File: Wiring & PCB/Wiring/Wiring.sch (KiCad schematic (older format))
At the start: 24 parts, among them M0 Motor_DC, M1 Motor_DC, M2 Stepper_Motor_unipolar_6pin, SW0 Ascention Limit 1, SW1 Ascention Limit 2, SW2 Declination Limit 1, U0 Arduino-mega, U1 Ardunio_Micro, U3 ULN2004A, U4 pchero_dualH

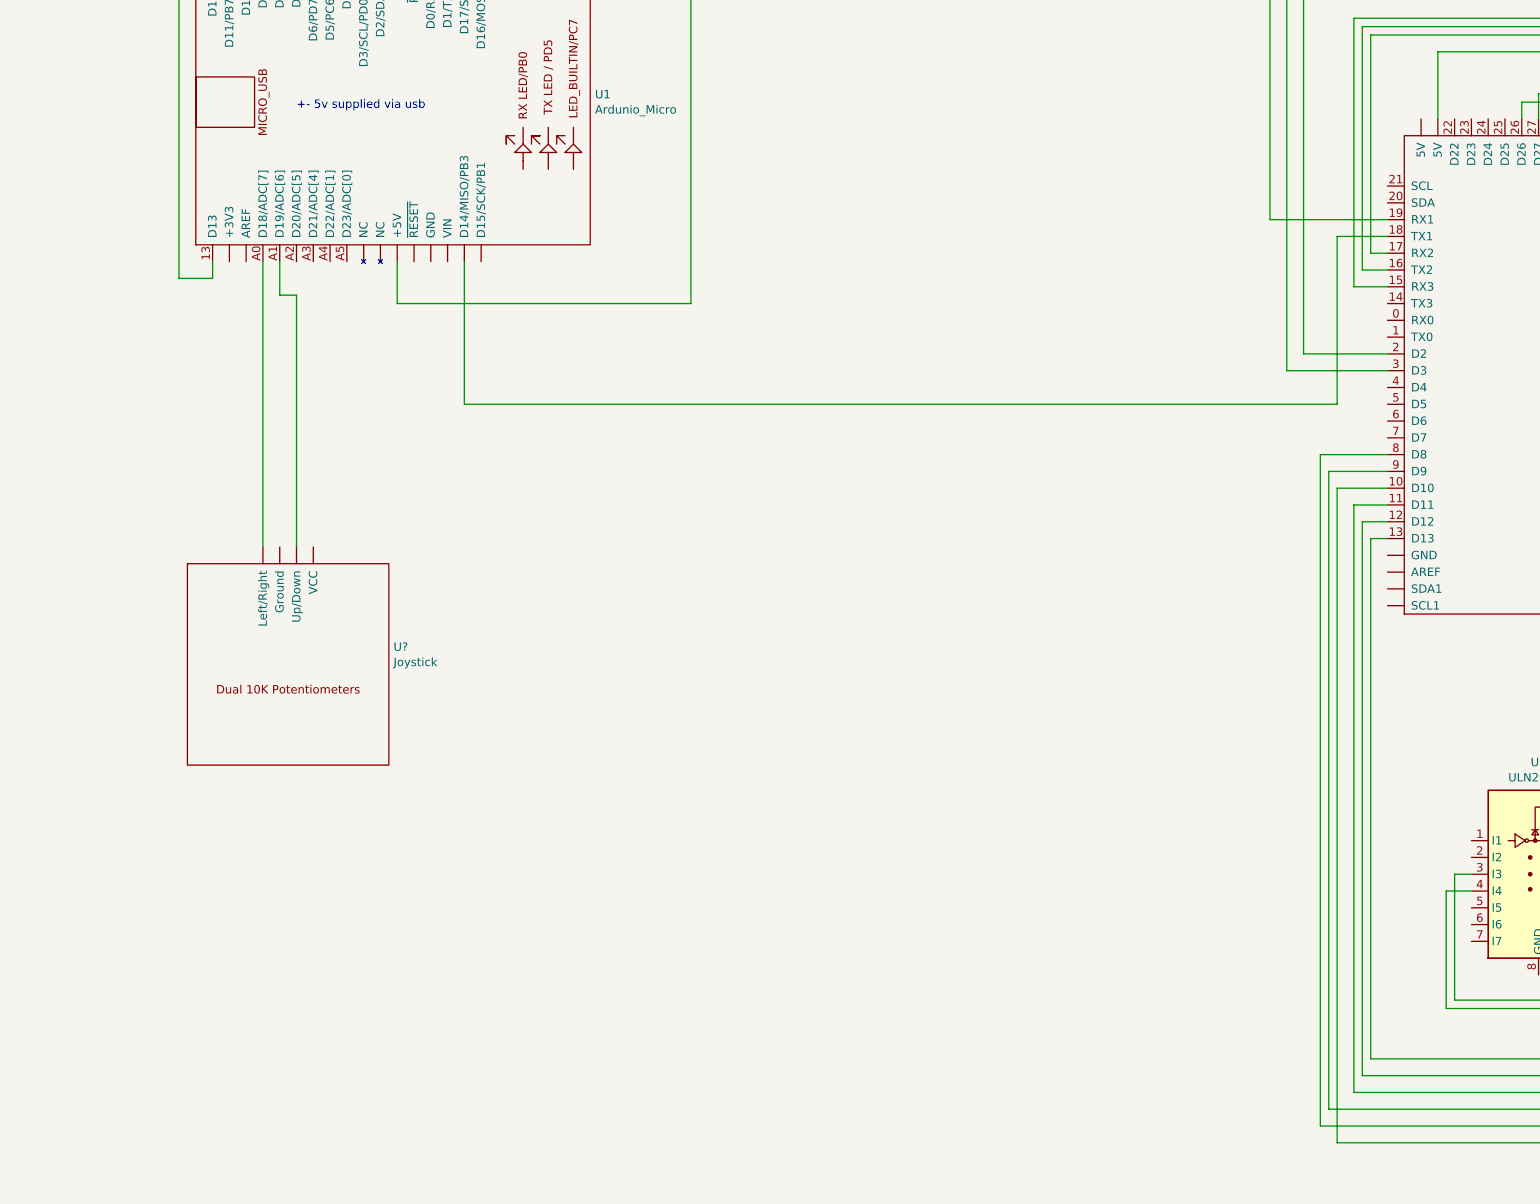
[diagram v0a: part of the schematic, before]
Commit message: chenges
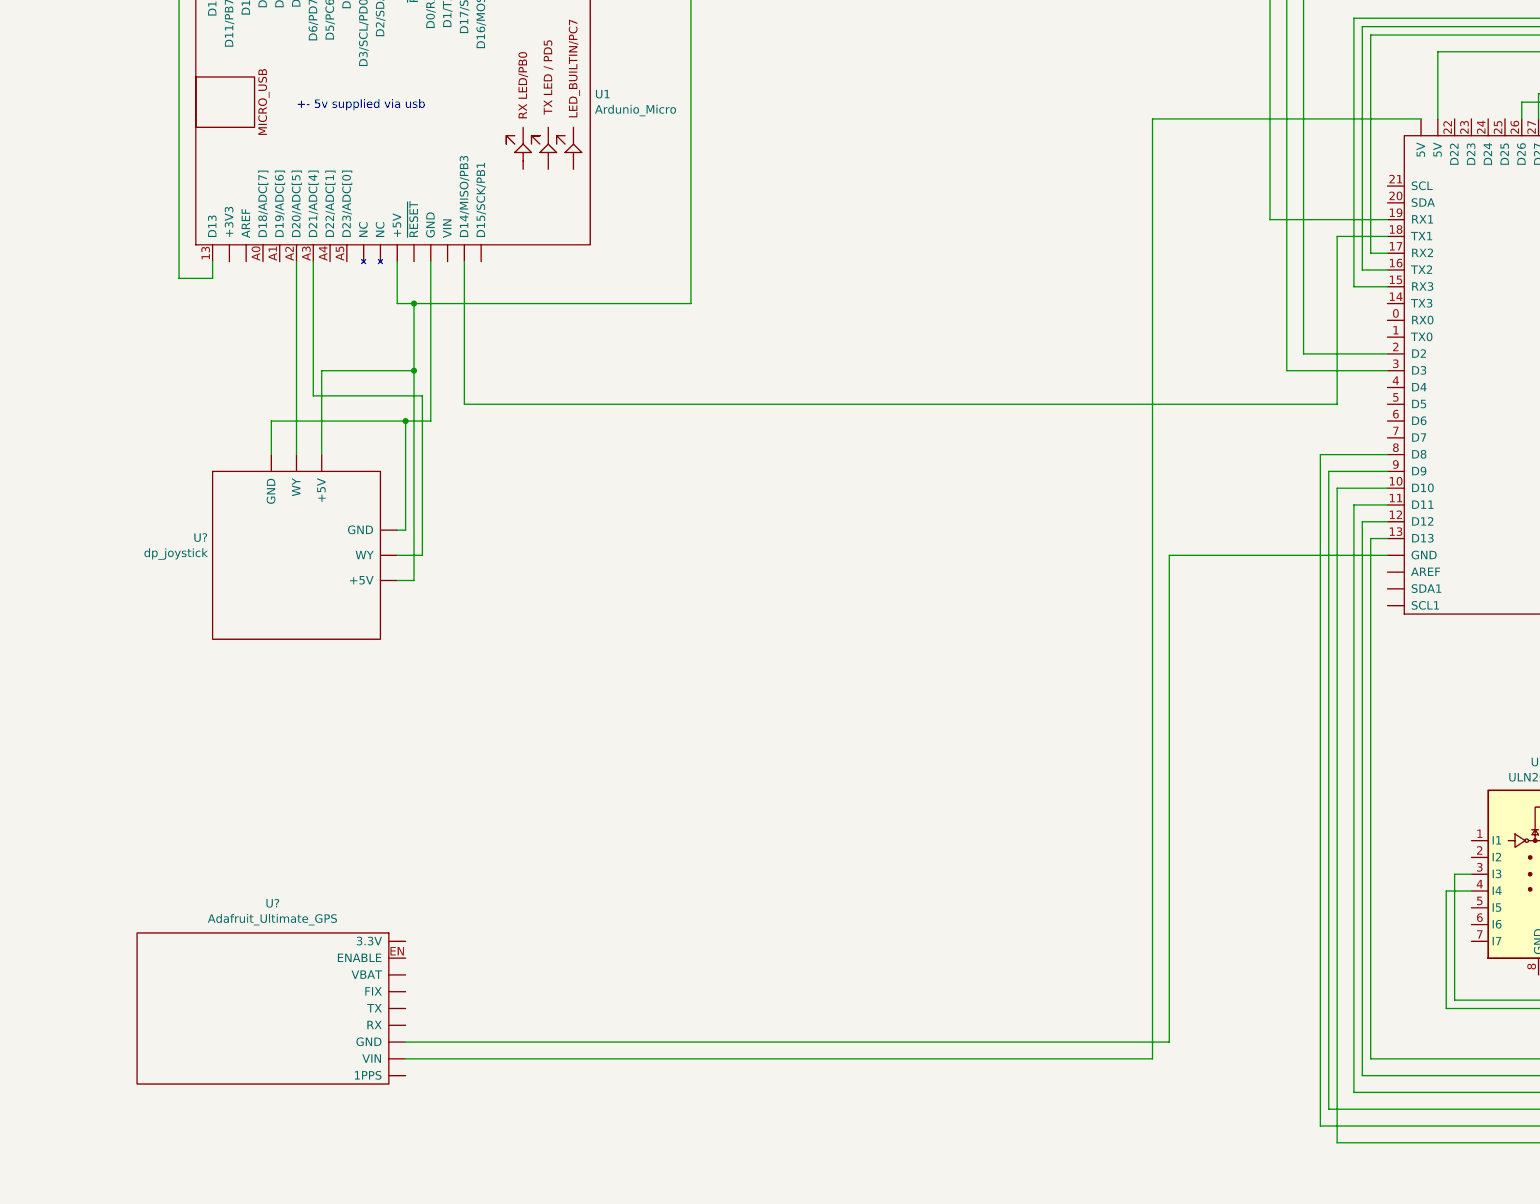
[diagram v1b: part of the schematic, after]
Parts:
- removed U?: Joystick, symbol Device:Joystick
- added U?: Adafruit_Ultimate_GPS, symbol Device:Adafruit_Ultimate_GPS
- added U?: dp_joystick, symbol Device:dp_joystick
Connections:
- net at U1.A2 (D20/ADC[5]): now also U?.~ (WY)
- net at U1.A3 (D21/ADC[4]): now also U?.~ (WY)
- net at U1.~ (~RESET): now also U?.~ (WY)
- net at RV?.1, SW?.1 (A), SW?.2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: now also U?.~ (WY)
- new net: U0.~ (VIN), U?.~ (VIN) (x2)
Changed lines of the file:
@@
 	3450 6900 3450 7150
 Wire Wire Line
-	3450 7150 5200 7150
+	3450 7150 3550 7150
 Wire Wire Line
 	5200 7150 5200 4300
@@
 	11500 11350 11500 10800
 $Comp
-L Device:Joystick U?
-U 1 1 5EE6A12F
-P 2800 9300
-F 0 "U?" H 3428 9404 50  0000 L CNN
-F 1 "Joystick" H 3428 9313 50  0000 L CNN
-F 2 "" H 2650 9300 50  0001 C CNN
-F 3 "" H 2650 9300 50  0001 C CNN
-	1    2800 9300
-	1    0    0    -1
-$EndComp
-Wire Wire Line
-	2650 6900 2650 8600
-Wire Wire Line
-	2850 8600 2850 7100
-Wire Wire Line
-	2850 7100 2750 7100
-Wire Wire Line
-	2750 7100 2750 6900
+L Device:Adafruit_Ultimate_GPS U?
+U 1 1 5EE87A51
+P 3400 11350
+F 0 "U?" V 2775 10658 50  0000 C CNN
+F 1 "Adafruit_Ultimate_GPS" V 2866 10658 50  0000 C CNN
+F 2 "" H 2950 9700 50  0001 C CNN
+F 3 "" H 2950 9700 50  0001 C CNN
+	1    3400 11350
+	0    1    1    0
+$EndComp
+Wire Wire Line
+	9550 6050 7950 6050
+Wire Wire Line
+	7950 6050 7950 11650
+Wire Wire Line
+	7950 11650 3500 11650
+Wire Wire Line
+	9350 8650 8050 8650
+Wire Wire Line
+	8050 8650 8050 11550
+Wire Wire Line
+	8050 11550 3500 11550
+$Comp
+L Device:dp_joystick U?
+U 1 1 5EF4B780
+P 2850 8650
+F 0 "U?" H 2322 8754 50  0000 R CNN
+F 1 "dp_joystick" H 2322 8663 50  0000 R CNN
+F 2 "" H 4350 9700 50  0001 C CNN
+F 3 "" H 4350 9700 50  0001 C CNN
+	1    2850 8650
+	1    0    0    -1
+$EndComp
+Wire Wire Line
+	2850 8050 2850 6900
+Wire Wire Line
+	3450 8650 3600 8650
+Wire Wire Line
+	3600 8650 3600 7700
+Wire Wire Line
+	3600 7700 2950 7700
+Wire Wire Line
+	2950 7700 2950 6900
+Wire Wire Line
+	2700 8050 2700 7850
+Wire Wire Line
+	2700 7850 3500 7850
+Wire Wire Line
+	3650 7850 3650 6900
+Wire Wire Line
+	3450 8500 3500 8500
+Wire Wire Line
+	3500 8500 3500 7850
+Connection ~ 3500 7850
+Wire Wire Line
+	3500 7850 3650 7850
+Wire Wire Line
+	3000 8050 3000 7550
+Wire Wire Line
+	3000 7550 3550 7550
+Wire Wire Line
+	3550 7550 3550 7150
+Connection ~ 3550 7150
+Wire Wire Line
+	3550 7150 5200 7150
+Wire Wire Line
+	3450 8800 3550 8800
+Wire Wire Line
+	3550 8800 3550 7550
+Connection ~ 3550 7550
 $EndSCHEMATC
